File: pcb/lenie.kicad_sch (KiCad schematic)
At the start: 3 parts, among them J1 Conn_01x05_MountingPin, U1 CR2013-MI2120, U2 ESP32-DEVKIT-V1

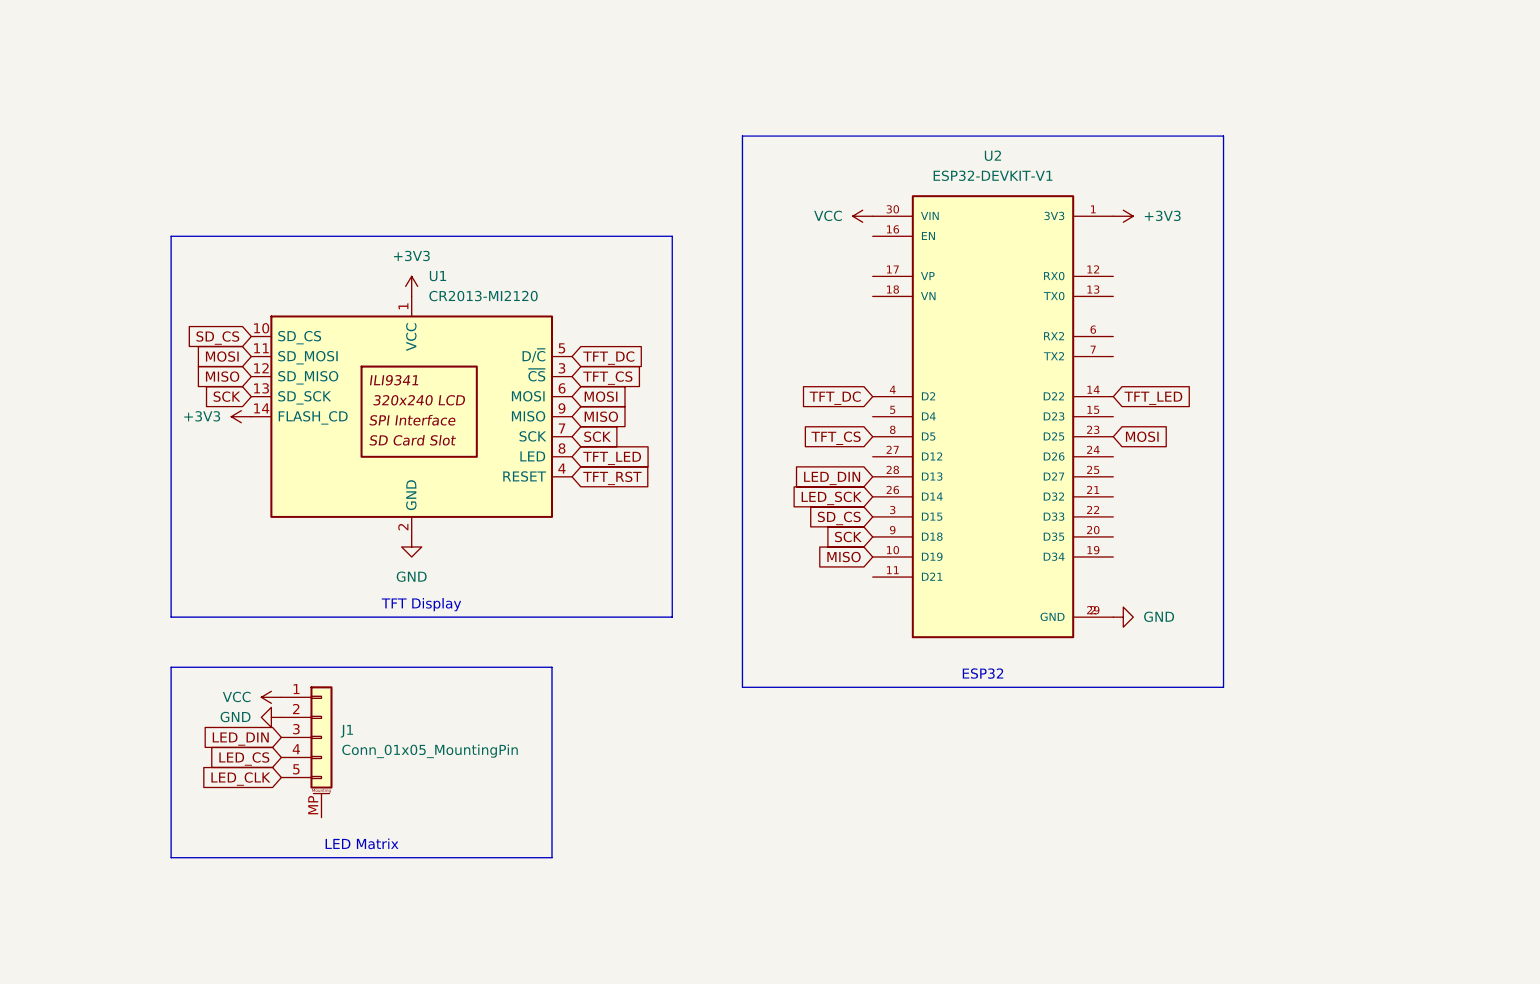
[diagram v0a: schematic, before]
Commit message: vault backup: 2025-05-28 22:00:58
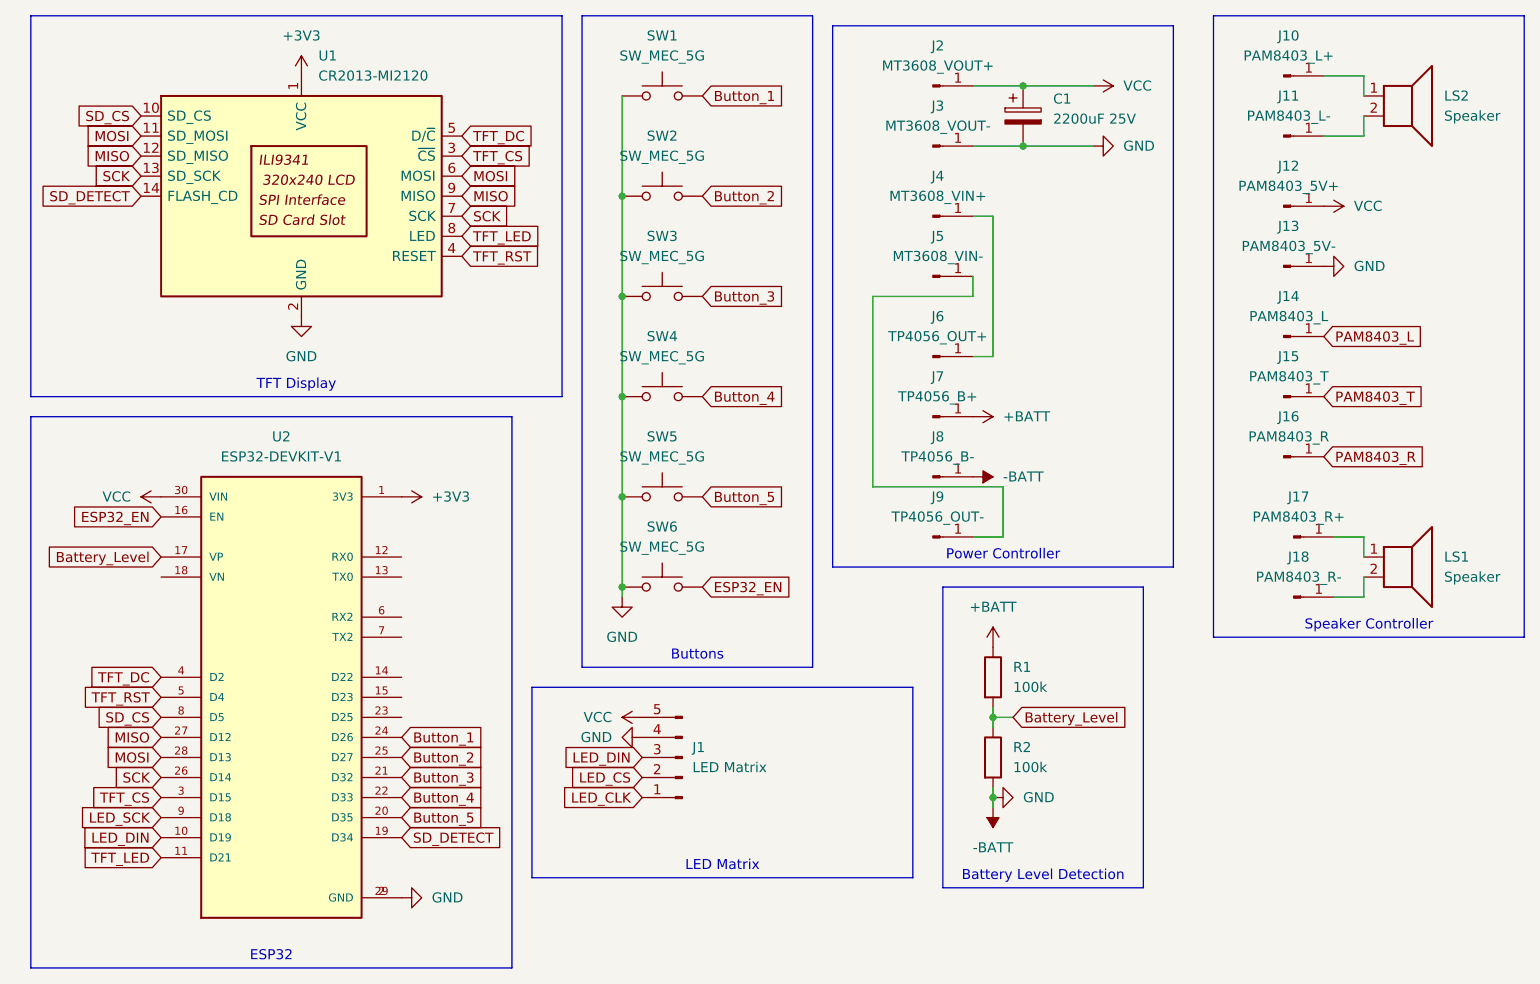
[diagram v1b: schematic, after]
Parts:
- removed J1: Conn_01x05_MountingPin, Connector_PinHeader_2.54mm:PinHeader_1x05_P2.54mm_Vertical, symbol Connector_Generic_MountingPin:Conn_01x05_MountingPin
- added C1: 2200uF 25V, PCM_Capacitor_THT_AKL:CP_Radial_D13.0mm_P5.00mm, symbol PCM_Capacitor_AKL:CP_Radial_D13.0mm_P5.00mm
- added J1: LED Matrix, symbol Connector:Conn_01x05_Pin
- added J10: PAM8403_L+, symbol Connector:Conn_01x01_Pin
- added J11: PAM8403_L-, symbol Connector:Conn_01x01_Pin
- added J12: PAM8403_5V+, symbol Connector:Conn_01x01_Pin
- added J13: PAM8403_5V-, symbol Connector:Conn_01x01_Pin
- added J14: PAM8403_L, symbol Connector:Conn_01x01_Pin
- added J15: PAM8403_T, symbol Connector:Conn_01x01_Pin
- added J16: PAM8403_R, symbol Connector:Conn_01x01_Pin
- added J17: PAM8403_R+, symbol Connector:Conn_01x01_Pin
- added J18: PAM8403_R-, symbol Connector:Conn_01x01_Pin
- added J2: MT3608_VOUT+, symbol Connector:Conn_01x01_Pin
- added J3: MT3608_VOUT-, symbol Connector:Conn_01x01_Pin
- added J4: MT3608_VIN+, symbol Connector:Conn_01x01_Pin
- added J5: MT3608_VIN-, symbol Connector:Conn_01x01_Pin
- added J6: TP4056_OUT+, symbol Connector:Conn_01x01_Pin
- added J7: TP4056_B+, symbol Connector:Conn_01x01_Pin
- added J8: TP4056_B-, symbol Connector:Conn_01x01_Pin
- added J9: TP4056_OUT-, symbol Connector:Conn_01x01_Pin
- added LS1, LS2: Speaker, symbol Device:Speaker
- added R1, R2: 100k, symbol Device:R
- added SW1, SW2, SW3, SW4, SW5, SW6: SW_MEC_5G, symbol Switch:SW_MEC_5G
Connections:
- net +3V3: no longer U1.14 (FLASH_CD)
- net LED_CLK: now also J1.1 (Pin_1)
- net LED_CS: now also J1.2 (Pin_2)
- net LED_DIN: now also U2.10 (D19), J1.3 (Pin_3); no longer U2.28 (D13)
- net LED_SCK: now also U2.9 (D18); no longer U2.26 (D14)
- net MISO: now also U2.27 (D12); no longer U2.10 (D19)
- net MOSI: now also U2.28 (D13); no longer U2.23 (D25)
- net SCK: now also U2.26 (D14); no longer U2.9 (D18)
- net SD_CS: now also U2.8 (D5); no longer U2.3 (D15)
- net TFT_CS: now also U2.3 (D15); no longer U2.8 (D5)
- net TFT_LED: now also U2.11 (D21); no longer U2.14 (D22)
- net TFT_RST: now also U2.5 (D4)
- net VCC: now also C1.1, J1.5 (Pin_5), J12.1 (Pin_1), J2.1 (Pin_1)
- net ESP32_EN: now reaches U2.16 (EN)
- net ESP32_EN: now also SW6.3 (B), SW6.4 (B)
- net Battery_Level: now reaches U2.17 (VP)
- net Battery_Level: now also R1.2, R2.1
- net SD_DETECT: now reaches U2.19 (D34)
- net SD_DETECT: now also U1.14 (FLASH_CD)
- net Button_5: now reaches U2.20 (D35)
- net Button_5: now also SW5.3 (B), SW5.4 (B)
- net Button_3: now reaches U2.21 (D32)
- net Button_3: now also SW3.3 (B), SW3.4 (B)
- net Button_4: now reaches U2.22 (D33)
- net Button_4: now also SW4.3 (B), SW4.4 (B)
- net Button_1: now reaches U2.24 (D26)
- net Button_1: now also SW1.3 (B), SW1.4 (B)
- net Button_2: now reaches U2.25 (D27)
- net Button_2: now also SW2.3 (B), SW2.4 (B)
- net GND renamed -BATT
- net -BATT: now also C1.2, J1.4 (Pin_4), J13.1 (Pin_1), J3.1 (Pin_1), J8.1 (Pin_1), R2.2, SW1.1 (A), SW1.2 (A), SW2.1 (A), SW2.2 (A), SW3.1 (A), SW3.2 (A), SW4.1 (A), SW4.2 (A), SW5.1 (A), SW5.2 (A), SW6.1 (A), SW6.2 (A)
- new net: J10.1 (Pin_1), LS2.1
- new net: J11.1 (Pin_1), LS2.2
- new net: J4.1 (Pin_1), J6.1 (Pin_1)
- new net: J18.1 (Pin_1), LS1.2
- new net: J5.1 (Pin_1), J9.1 (Pin_1)
- new net: J17.1 (Pin_1), LS1.1
- new net +BATT: J7.1 (Pin_1), R1.1
- new net PAM8403_L: J14.1 (Pin_1)
- new net PAM8403_R: J16.1 (Pin_1)
- new net PAM8403_T: J15.1 (Pin_1)
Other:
- title: (none) -> Lenie
- moved on the sheet: U1, U2
